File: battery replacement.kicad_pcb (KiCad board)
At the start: 2 copper layers, 25 x 9 mm, 16 parts, among them U1 RT5788BGJ8F, U2 Y4203-ADJM6R

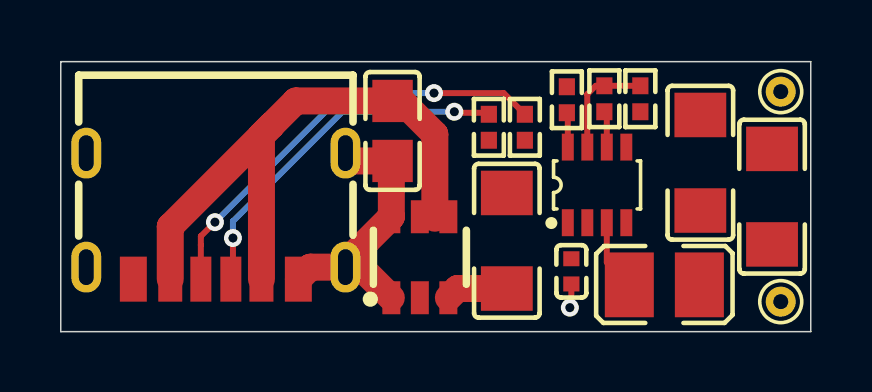
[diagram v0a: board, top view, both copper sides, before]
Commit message: kicad prelim version
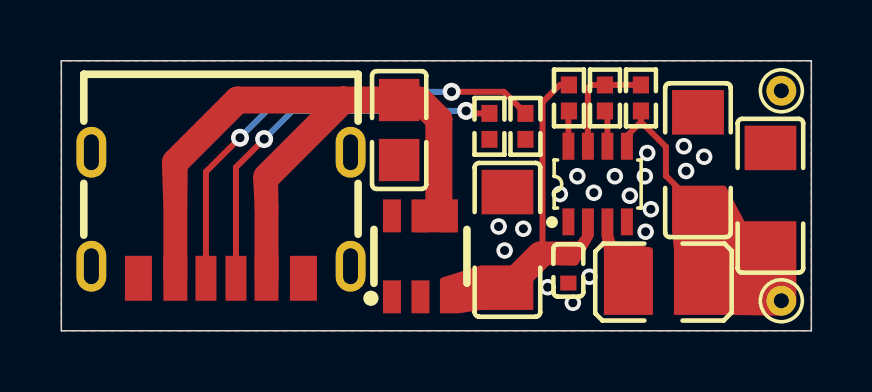
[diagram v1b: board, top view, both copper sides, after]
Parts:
- moved C1 0.22 mm to (143.3, 68.4)
- moved USB1 0.17 mm to (137.4, 71.2)
- moved C4 0.12 mm to (153.3, 69.4)
- moved C3 0.10 mm to (148.9, 73.1)
- moved R3 0.09 mm to (149.0, 67.3)
- moved L1 0.09 mm to (152.1, 73.5)
- moved C5 0.06 mm to (155.7, 70.6)
- renumbered C7 to C1, C1 to C2, C2 to C3, C3 to C4, C4 to C5, R5 to R1, R6 to R2, R2 to R4, R1 to R5, U2 to U1, U1 to U2
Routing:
- net GND: track 11.6 -> 1.21 mm, vias 1 -> 18
- net +5V: track 2.08 -> 7.78 mm
- net /VOUT: track 0.00 -> 5.05 mm
- net /LX: track 2.38 -> 0.00 mm
- net Net-(USB1-CC1): track 14.5 -> 15.6 mm
- net Net-(USB1-CC2): track 12.0 -> 13.0 mm
- added copper zone on B.Cu, net GND
- added copper zone on F.Cu, net GND
